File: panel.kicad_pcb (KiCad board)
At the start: 2 copper layers, 104 x 99 mm, 192 parts, among them J1 USB, J2 UART, U1 CH340X, U2 AMS1117-3.3

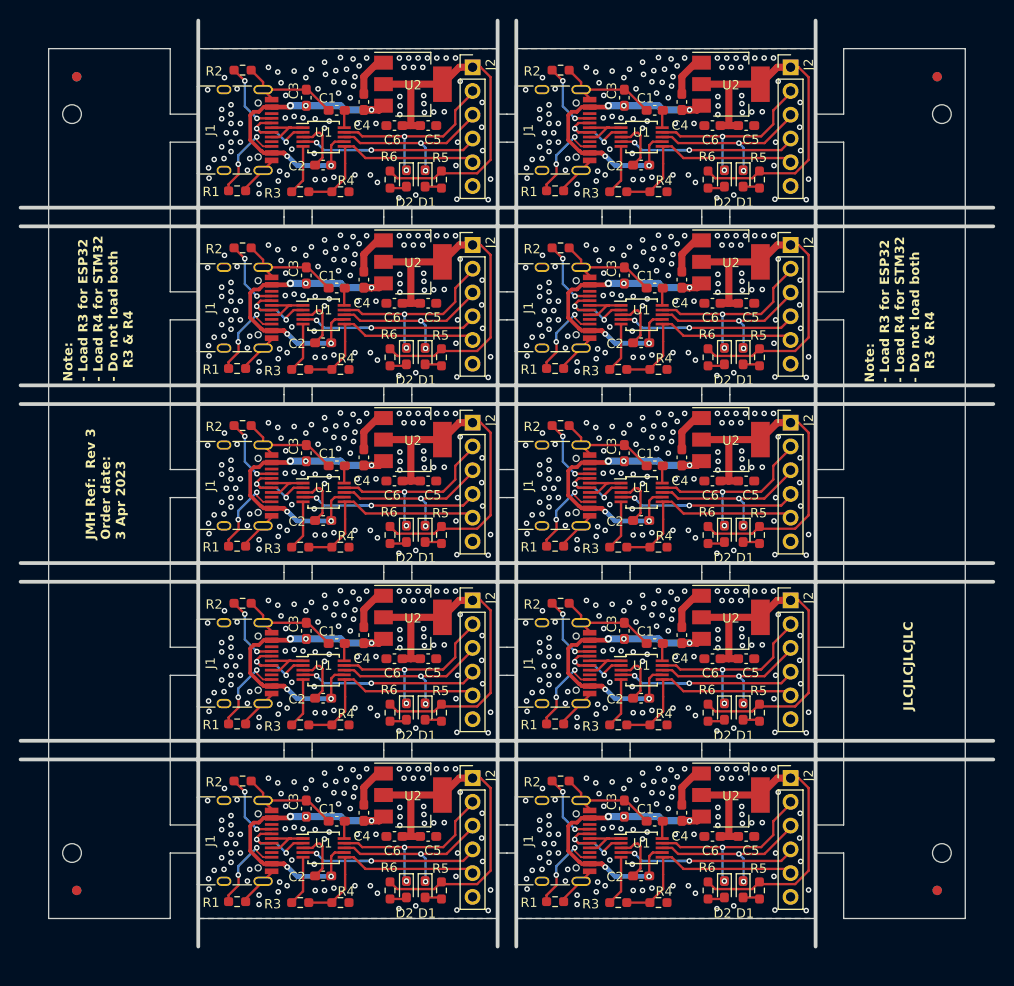
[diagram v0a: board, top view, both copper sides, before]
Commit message: Rev 5
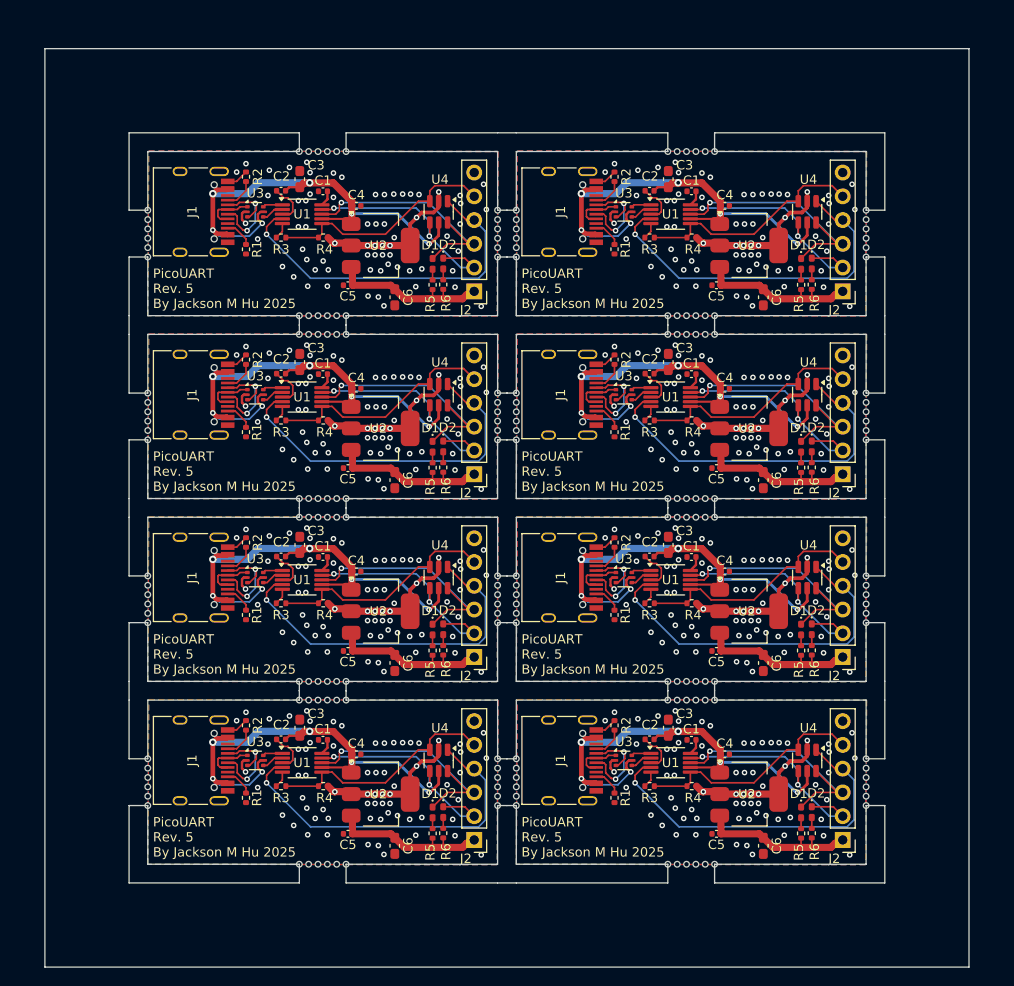
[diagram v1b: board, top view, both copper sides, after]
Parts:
- removed the C1 at (130.3, 64.6)
- removed the C1 at (130.3, 83.6)
- removed the C1 at (164.3, 102.6)
- removed the C1 at (164.3, 26.6)
- removed the C1 at (130.3, 102.6)
- removed the C1 at (130.3, 26.6)
- removed the C1 at (130.3, 45.6)
- removed the C1 at (164.3, 83.6)
- removed the C1 at (164.3, 45.6)
- removed the C1 at (164.3, 64.6)
- removed the C2 at (162.8, 70.5)
- removed the C2 at (128.8, 51.5)
- removed the C2 at (128.8, 70.5)
- removed the C2 at (162.8, 32.5)
- removed the C2 at (162.8, 108.5)
- removed the C2 at (128.8, 108.5)
- removed the C2 at (128.8, 32.5)
- removed the C2 at (128.8, 89.5)
- removed the C2 at (162.8, 51.5)
- removed the C2 at (162.8, 89.5)
- removed the C3 at (127.0, 25.2)
- removed the C3 at (127.0, 82.2)
- removed the C3 at (161.1, 44.2)
- removed the C3 at (127.0, 101.2)
- removed the C3 at (127.0, 63.2)
- removed the C3 at (161.1, 63.2)
- removed the C3 at (161.1, 82.2)
- removed the C3 at (161.1, 101.2)
- removed the C3 at (161.1, 25.2)
- removed the C3 at (127.0, 44.2)
- removed the C4 at (133.2, 25.7)
- removed the C4 at (133.2, 82.7)
- removed the C4 at (167.2, 44.7)
- removed the C4 at (133.2, 101.7)
- removed the C4 at (133.2, 63.7)
- removed the C4 at (167.2, 63.7)
- removed the C4 at (167.2, 82.7)
- removed the C4 at (167.2, 101.7)
- removed the C4 at (167.2, 25.7)
- removed the C4 at (133.2, 44.7)
- removed the C5 at (174.1, 47.2)
- removed the C5 at (140.1, 85.2)
- removed the C5 at (140.1, 104.2)
- removed the C5 at (140.1, 28.2)
- removed the C5 at (140.1, 66.2)
- removed the C5 at (174.1, 66.2)
- removed the C5 at (174.1, 85.2)
- removed the C5 at (174.1, 104.2)
- removed the C5 at (174.1, 28.2)
- removed the C5 at (140.1, 47.2)
- removed the C6 at (136.5, 28.2)
- removed the C6 at (136.5, 85.2)
- removed the C6 at (170.5, 47.2)
- removed the C6 at (136.5, 104.2)
- removed the C6 at (136.5, 66.2)
- removed the C6 at (170.5, 66.2)
- removed the C6 at (170.5, 85.2)
- removed the C6 at (170.5, 104.2)
- removed the C6 at (170.5, 28.2)
- removed the C6 at (136.5, 47.2)
- removed the D1 at (139.8, 33.9)
- removed the D1 at (139.8, 90.9)
- removed the D1 at (173.8, 52.9)
- removed the D1 at (139.8, 109.9)
- removed the D1 at (139.8, 71.9)
- removed the D1 at (173.8, 71.9)
- removed the D1 at (173.8, 90.9)
- removed the D1 at (173.8, 109.9)
- removed the D1 at (173.8, 33.9)
- removed the D1 at (139.8, 52.9)
- removed the D2 at (137.8, 33.9)
- removed the D2 at (137.8, 90.9)
- removed the D2 at (171.8, 52.9)
- removed the D2 at (137.8, 109.9)
- removed the D2 at (137.8, 71.9)
- removed the D2 at (171.8, 71.9)
- removed the D2 at (171.8, 90.9)
- removed the D2 at (171.8, 109.9)
- removed the D2 at (171.8, 33.9)
- removed the D2 at (137.8, 52.9)
- removed the J1 at (119.3, 28.7)
- removed the J1 at (119.3, 85.7)
- removed the J1 at (153.3, 47.7)
- removed the J1 at (119.3, 104.7)
- removed the J1 at (119.3, 66.7)
- removed the J1 at (153.3, 66.7)
- removed the J1 at (153.3, 85.7)
- removed the J1 at (153.3, 104.7)
- removed the J1 at (153.3, 28.7)
- removed the J1 at (119.3, 47.7)
- removed the J2 at (144.8, 22.0)
- removed the J2 at (144.8, 79.0)
- removed the J2 at (178.8, 41.0)
- removed the J2 at (144.8, 98.0)
- removed the J2 at (178.8, 22.0)
- removed the J2 at (144.8, 60.0)
- removed the J2 at (178.8, 60.0)
- removed the J2 at (178.8, 79.0)
- removed the J2 at (178.8, 98.0)
- removed the J2 at (144.8, 41.0)
- removed the R1 at (119.7, 35.2)
- removed the R1 at (119.7, 92.2)
- removed the R1 at (153.7, 54.2)
- removed the R1 at (119.7, 111.2)
- removed the R1 at (119.7, 73.2)
- removed the R1 at (153.7, 73.2)
- removed the R1 at (153.7, 92.2)
- removed the R1 at (153.7, 111.2)
- removed the R1 at (153.7, 35.2)
- removed the R1 at (119.7, 54.2)
- removed the R2 at (120.2, 22.3)
- removed the R2 at (120.2, 79.3)
- removed the R2 at (154.2, 41.3)
- removed the R2 at (120.2, 98.3)
- removed the R2 at (120.2, 60.3)
- removed the R2 at (154.2, 60.3)
- removed the R2 at (154.2, 79.3)
- removed the R2 at (154.2, 98.3)
- removed the R2 at (154.2, 22.3)
- removed the R2 at (120.2, 41.3)
- removed the R3 at (126.4, 35.3)
- removed the R3 at (126.4, 92.3)
- removed the R3 at (160.4, 54.3)
- removed the R3 at (126.4, 111.3)
- removed the R3 at (126.4, 73.3)
- removed the R3 at (160.4, 73.3)
- removed the R3 at (160.4, 92.3)
- removed the R3 at (160.4, 111.3)
- removed the R3 at (160.4, 35.3)
- removed the R3 at (126.4, 54.3)
- removed the R4 at (130.7, 35.3)
- removed the R4 at (130.7, 92.3)
- removed the R4 at (164.7, 54.3)
- removed the R4 at (130.7, 111.3)
- removed the R4 at (130.7, 73.3)
- removed the R4 at (164.7, 73.3)
- removed the R4 at (164.7, 92.3)
- removed the R4 at (164.7, 111.3)
- removed the R4 at (164.7, 35.3)
- removed the R4 at (130.7, 54.3)
- removed the R5 at (141.5, 34.0)
- removed the R5 at (141.5, 91.0)
- removed the R5 at (175.5, 53.0)
- removed the R5 at (141.5, 110.0)
- removed the R5 at (141.5, 72.0)
- removed the R5 at (175.5, 72.0)
- removed the R5 at (175.5, 91.0)
- removed the R5 at (175.5, 110.0)
- removed the R5 at (175.5, 34.0)
- removed the R5 at (141.5, 53.0)
- removed the R6 at (136.0, 34.0)
- removed the R6 at (136.0, 91.0)
- removed the R6 at (170.0, 53.0)
- removed the R6 at (136.0, 110.0)
- removed the R6 at (136.0, 72.0)
- removed the R6 at (170.0, 72.0)
- removed the R6 at (170.0, 91.0)
- removed the R6 at (170.0, 110.0)
- removed the R6 at (170.0, 34.0)
- removed the R6 at (136.0, 53.0)
- removed REF** (x8): Fiducial, Fiducial
- removed REF** (x4): NPTH, NPTH
- removed the U1 at (128.9, 105.5)
- removed the U1 at (162.9, 48.5)
- removed the U1 at (128.9, 67.5)
- removed the U1 at (162.9, 67.5)
- removed the U1 at (162.9, 86.5)
- removed the U1 at (128.9, 48.5)
- removed the U1 at (128.9, 86.5)
- removed the U1 at (162.9, 105.5)
- removed the U1 at (162.9, 29.4)
- removed the U1 at (128.9, 29.4)
- removed the U2 at (138.4, 23.8)
- removed the U2 at (138.4, 80.8)
- removed the U2 at (172.4, 42.8)
- removed the U2 at (138.4, 99.8)
- removed the U2 at (138.4, 61.8)
- removed the U2 at (172.4, 61.8)
- removed the U2 at (172.4, 80.8)
- removed the U2 at (172.4, 99.8)
- removed the U2 at (172.4, 23.8)
- removed the U2 at (138.4, 42.8)
- added C1: 100nF, Capacitor_SMD:C_0402_1005Metric, F.Cu at (128.8, 74.3)
- added C1: 100nF, Capacitor_SMD:C_0402_1005Metric, F.Cu at (128.8, 93.9)
- added C1: 100nF, Capacitor_SMD:C_0402_1005Metric, F.Cu at (168.2, 93.9)
- added C1: 100nF, Capacitor_SMD:C_0402_1005Metric, F.Cu at (168.2, 74.3)
- added C1: 100nF, Capacitor_SMD:C_0402_1005Metric, F.Cu at (168.2, 54.8)
- added C1: 100nF, Capacitor_SMD:C_0402_1005Metric, F.Cu at (168.2, 35.2)
- added C1: 100nF, Capacitor_SMD:C_0402_1005Metric, F.Cu at (128.8, 35.2)
- added C1: 100nF, Capacitor_SMD:C_0402_1005Metric, F.Cu at (128.8, 54.8)
- added C2: 100nF, Capacitor_SMD:C_0402_1005Metric, F.Cu at (163.8, 54.8)
- added C2: 100nF, Capacitor_SMD:C_0402_1005Metric, F.Cu at (163.8, 93.8)
- added C2: 100nF, Capacitor_SMD:C_0402_1005Metric, F.Cu at (163.8, 35.2)
- added C2: 100nF, Capacitor_SMD:C_0402_1005Metric, F.Cu at (124.3, 93.8)
- added C2: 100nF, Capacitor_SMD:C_0402_1005Metric, F.Cu at (124.3, 35.2)
- added C2: 100nF, Capacitor_SMD:C_0402_1005Metric, F.Cu at (124.3, 54.8)
- added C2: 100nF, Capacitor_SMD:C_0402_1005Metric, F.Cu at (163.8, 74.3)
- added C2: 100nF, Capacitor_SMD:C_0402_1005Metric, F.Cu at (124.3, 74.3)
- added C3: 10uF, Capacitor_SMD:C_0603_1608Metric_Pad1.08x0.95mm_HandSolder, F.Cu at (126.3, 53.5)
- added C3: 10uF, Capacitor_SMD:C_0603_1608Metric_Pad1.08x0.95mm_HandSolder, F.Cu at (165.8, 73.0)
- added C3: 10uF, Capacitor_SMD:C_0603_1608Metric_Pad1.08x0.95mm_HandSolder, F.Cu at (126.3, 73.0)
- added C3: 10uF, Capacitor_SMD:C_0603_1608Metric_Pad1.08x0.95mm_HandSolder, F.Cu at (165.8, 92.6)
- added C3: 10uF, Capacitor_SMD:C_0603_1608Metric_Pad1.08x0.95mm_HandSolder, F.Cu at (165.8, 34.0)
- added C3: 10uF, Capacitor_SMD:C_0603_1608Metric_Pad1.08x0.95mm_HandSolder, F.Cu at (126.3, 34.0)
- added C3: 10uF, Capacitor_SMD:C_0603_1608Metric_Pad1.08x0.95mm_HandSolder, F.Cu at (126.3, 92.6)
- added C3: 10uF, Capacitor_SMD:C_0603_1608Metric_Pad1.08x0.95mm_HandSolder, F.Cu at (165.8, 53.5)
- added C4: 0.1uF, Capacitor_SMD:C_0402_1005Metric, F.Cu at (171.8, 36.8)
- added C4: 0.1uF, Capacitor_SMD:C_0402_1005Metric, F.Cu at (132.4, 95.5)
- added C4: 0.1uF, Capacitor_SMD:C_0402_1005Metric, F.Cu at (132.4, 36.8)
- added C4: 0.1uF, Capacitor_SMD:C_0402_1005Metric, F.Cu at (132.4, 75.9)
- added C4: 0.1uF, Capacitor_SMD:C_0402_1005Metric, F.Cu at (171.8, 95.5)
- added C4: 0.1uF, Capacitor_SMD:C_0402_1005Metric, F.Cu at (171.8, 56.4)
- added C4: 0.1uF, Capacitor_SMD:C_0402_1005Metric, F.Cu at (171.8, 75.9)
- added C4: 0.1uF, Capacitor_SMD:C_0402_1005Metric, F.Cu at (132.4, 56.4)
- added C5: 0.1uF, Capacitor_SMD:C_0402_1005Metric, F.Cu at (170.9, 64.8)
- added C5: 0.1uF, Capacitor_SMD:C_0402_1005Metric, F.Cu at (131.5, 104.0)
- added C5: 0.1uF, Capacitor_SMD:C_0402_1005Metric, F.Cu at (131.5, 45.3)
- added C5: 0.1uF, Capacitor_SMD:C_0402_1005Metric, F.Cu at (170.9, 104.0)
- added C5: 0.1uF, Capacitor_SMD:C_0402_1005Metric, F.Cu at (170.9, 45.3)
- added C5: 0.1uF, Capacitor_SMD:C_0402_1005Metric, F.Cu at (131.5, 64.8)
- added C5: 0.1uF, Capacitor_SMD:C_0402_1005Metric, F.Cu at (131.5, 84.4)
- added C5: 0.1uF, Capacitor_SMD:C_0402_1005Metric, F.Cu at (170.9, 84.4)
- added C6: 10uF, Capacitor_SMD:C_0603_1608Metric_Pad1.08x0.95mm_HandSolder, F.Cu at (136.5, 105.2)
- added C6: 10uF, Capacitor_SMD:C_0603_1608Metric_Pad1.08x0.95mm_HandSolder, F.Cu at (136.5, 46.6)
- added C6: 10uF, Capacitor_SMD:C_0603_1608Metric_Pad1.08x0.95mm_HandSolder, F.Cu at (175.9, 85.7)
- added C6: 10uF, Capacitor_SMD:C_0603_1608Metric_Pad1.08x0.95mm_HandSolder, F.Cu at (136.5, 66.1)
- added C6: 10uF, Capacitor_SMD:C_0603_1608Metric_Pad1.08x0.95mm_HandSolder, F.Cu at (136.5, 85.7)
- added C6: 10uF, Capacitor_SMD:C_0603_1608Metric_Pad1.08x0.95mm_HandSolder, F.Cu at (175.9, 105.2)
- added C6: 10uF, Capacitor_SMD:C_0603_1608Metric_Pad1.08x0.95mm_HandSolder, F.Cu at (175.9, 46.6)
- added C6: 10uF, Capacitor_SMD:C_0603_1608Metric_Pad1.08x0.95mm_HandSolder, F.Cu at (175.9, 66.1)
- added D1: LED, LED_SMD:LED_0402_1005Metric_Pad0.77x0.64mm_HandSolder, F.Cu at (140.6, 82.1)
- added D1: LED, LED_SMD:LED_0402_1005Metric_Pad0.77x0.64mm_HandSolder, F.Cu at (179.9, 43.0)
- added D1: LED, LED_SMD:LED_0402_1005Metric_Pad0.77x0.64mm_HandSolder, F.Cu at (179.9, 101.7)
- added D1: LED, LED_SMD:LED_0402_1005Metric_Pad0.77x0.64mm_HandSolder, F.Cu at (140.6, 62.6)
- added D1: LED, LED_SMD:LED_0402_1005Metric_Pad0.77x0.64mm_HandSolder, F.Cu at (140.6, 101.7)
- added D1: LED, LED_SMD:LED_0402_1005Metric_Pad0.77x0.64mm_HandSolder, F.Cu at (179.9, 82.1)
- added D1: LED, LED_SMD:LED_0402_1005Metric_Pad0.77x0.64mm_HandSolder, F.Cu at (179.9, 62.6)
- added D1: LED, LED_SMD:LED_0402_1005Metric_Pad0.77x0.64mm_HandSolder, F.Cu at (140.6, 43.0)
- added D2: LED, LED_SMD:LED_0402_1005Metric_Pad0.77x0.64mm_HandSolder, F.Cu at (181.1, 101.6)
- added D2: LED, LED_SMD:LED_0402_1005Metric_Pad0.77x0.64mm_HandSolder, F.Cu at (181.1, 43.0)
- added D2: LED, LED_SMD:LED_0402_1005Metric_Pad0.77x0.64mm_HandSolder, F.Cu at (141.7, 101.6)
- added D2: LED, LED_SMD:LED_0402_1005Metric_Pad0.77x0.64mm_HandSolder, F.Cu at (141.7, 82.1)
- added D2: LED, LED_SMD:LED_0402_1005Metric_Pad0.77x0.64mm_HandSolder, F.Cu at (181.1, 62.5)
- added D2: LED, LED_SMD:LED_0402_1005Metric_Pad0.77x0.64mm_HandSolder, F.Cu at (181.1, 82.1)
- added D2: LED, LED_SMD:LED_0402_1005Metric_Pad0.77x0.64mm_HandSolder, F.Cu at (141.7, 62.5)
- added D2: LED, LED_SMD:LED_0402_1005Metric_Pad0.77x0.64mm_HandSolder, F.Cu at (141.7, 43.0)
- added J1: USB, Connector_USB:USB_C_Receptacle_HRO_TYPE-C-31-M-12, F.Cu at (114.6, 57.0)
- added J1: USB, Connector_USB:USB_C_Receptacle_HRO_TYPE-C-31-M-12, F.Cu at (154.0, 96.1)
- added J1: USB, Connector_USB:USB_C_Receptacle_HRO_TYPE-C-31-M-12, F.Cu at (154.0, 37.5)
- added J1: USB, Connector_USB:USB_C_Receptacle_HRO_TYPE-C-31-M-12, F.Cu at (154.0, 76.5)
- added J1: USB, Connector_USB:USB_C_Receptacle_HRO_TYPE-C-31-M-12, F.Cu at (154.0, 57.0)
- added J1: USB, Connector_USB:USB_C_Receptacle_HRO_TYPE-C-31-M-12, F.Cu at (114.6, 37.5)
- added J1: USB, Connector_USB:USB_C_Receptacle_HRO_TYPE-C-31-M-12, F.Cu at (114.6, 76.5)
- added J1: USB, Connector_USB:USB_C_Receptacle_HRO_TYPE-C-31-M-12, F.Cu at (114.6, 96.1)
- added J2: UART, Connector_PinHeader_2.54mm:PinHeader_1x06_P2.54mm_Vertical, F.Cu at (184.4, 46.0)
- added J2: UART, Connector_PinHeader_2.54mm:PinHeader_1x06_P2.54mm_Vertical, F.Cu at (184.4, 65.5)
- added J2: UART, Connector_PinHeader_2.54mm:PinHeader_1x06_P2.54mm_Vertical, F.Cu at (145.0, 104.6)
- added J2: UART, Connector_PinHeader_2.54mm:PinHeader_1x06_P2.54mm_Vertical, F.Cu at (145.0, 85.0)
- added J2: UART, Connector_PinHeader_2.54mm:PinHeader_1x06_P2.54mm_Vertical, F.Cu at (145.0, 46.0)
- added J2: UART, Connector_PinHeader_2.54mm:PinHeader_1x06_P2.54mm_Vertical, F.Cu at (184.4, 85.0)
- added J2: UART, Connector_PinHeader_2.54mm:PinHeader_1x06_P2.54mm_Vertical, F.Cu at (145.0, 65.5)
- added J2: UART, Connector_PinHeader_2.54mm:PinHeader_1x06_P2.54mm_Vertical, F.Cu at (184.4, 104.6)
- added KiKit_MB_10_1: NPTH, NPTH, F.Cu at (147.5, 56.8)
- added KiKit_MB_10_2: NPTH, NPTH, F.Cu at (147.5, 57.8)
- added KiKit_MB_10_3: NPTH, NPTH, F.Cu at (147.5, 58.8)
- added KiKit_MB_10_4: NPTH, NPTH, F.Cu at (147.5, 59.8)
- added KiKit_MB_10_5: NPTH, NPTH, F.Cu at (147.5, 60.8)
- added KiKit_MB_10_6: NPTH, NPTH, F.Cu at (147.5, 61.8)
- added KiKit_MB_11_1: NPTH, NPTH, F.Cu at (126.3, 50.5)
- added KiKit_MB_11_2: NPTH, NPTH, F.Cu at (127.3, 50.5)
- added KiKit_MB_11_3: NPTH, NPTH, F.Cu at (128.3, 50.5)
- added KiKit_MB_11_4: NPTH, NPTH, F.Cu at (129.3, 50.5)
- added KiKit_MB_11_5: NPTH, NPTH, F.Cu at (130.3, 50.5)
- added KiKit_MB_11_6: NPTH, NPTH, F.Cu at (131.3, 50.5)
- added KiKit_MB_12_1: NPTH, NPTH, F.Cu at (131.3, 68.1)
- added KiKit_MB_12_2: NPTH, NPTH, F.Cu at (130.3, 68.1)
- added KiKit_MB_12_3: NPTH, NPTH, F.Cu at (129.3, 68.1)
- added KiKit_MB_12_4: NPTH, NPTH, F.Cu at (128.3, 68.1)
- added KiKit_MB_12_5: NPTH, NPTH, F.Cu at (127.3, 68.1)
- added KiKit_MB_12_6: NPTH, NPTH, F.Cu at (126.3, 68.1)
- added KiKit_MB_13_1: NPTH, NPTH, F.Cu at (149.5, 61.8)
- added KiKit_MB_13_2: NPTH, NPTH, F.Cu at (149.5, 60.8)
- added KiKit_MB_13_3: NPTH, NPTH, F.Cu at (149.5, 59.8)
- added KiKit_MB_13_4: NPTH, NPTH, F.Cu at (149.5, 58.8)
- added KiKit_MB_13_5: NPTH, NPTH, F.Cu at (149.5, 57.8)
- added KiKit_MB_13_6: NPTH, NPTH, F.Cu at (149.5, 56.8)
- added KiKit_MB_14_1: NPTH, NPTH, F.Cu at (186.9, 56.8)
- added KiKit_MB_14_2: NPTH, NPTH, F.Cu at (186.9, 57.8)
- added KiKit_MB_14_3: NPTH, NPTH, F.Cu at (186.9, 58.8)
- added KiKit_MB_14_4: NPTH, NPTH, F.Cu at (186.9, 59.8)
- added KiKit_MB_14_5: NPTH, NPTH, F.Cu at (186.9, 60.8)
- added KiKit_MB_14_6: NPTH, NPTH, F.Cu at (186.9, 61.8)
- added KiKit_MB_15_1: NPTH, NPTH, F.Cu at (165.7, 50.5)
- added KiKit_MB_15_2: NPTH, NPTH, F.Cu at (166.7, 50.5)
- added KiKit_MB_15_3: NPTH, NPTH, F.Cu at (167.7, 50.5)
- added KiKit_MB_15_4: NPTH, NPTH, F.Cu at (168.7, 50.5)
- added KiKit_MB_15_5: NPTH, NPTH, F.Cu at (169.7, 50.5)
- added KiKit_MB_15_6: NPTH, NPTH, F.Cu at (170.7, 50.5)
- added KiKit_MB_16_1: NPTH, NPTH, F.Cu at (170.7, 68.1)
- added KiKit_MB_16_2: NPTH, NPTH, F.Cu at (169.7, 68.1)
- added KiKit_MB_16_3: NPTH, NPTH, F.Cu at (168.7, 68.1)
- added KiKit_MB_16_4: NPTH, NPTH, F.Cu at (167.7, 68.1)
- added KiKit_MB_16_5: NPTH, NPTH, F.Cu at (166.7, 68.1)
- added KiKit_MB_16_6: NPTH, NPTH, F.Cu at (165.7, 68.1)
- added KiKit_MB_17_1: NPTH, NPTH, F.Cu at (110.1, 81.4)
- added KiKit_MB_17_2: NPTH, NPTH, F.Cu at (110.1, 80.4)
- added KiKit_MB_17_3: NPTH, NPTH, F.Cu at (110.1, 79.4)
- added KiKit_MB_17_4: NPTH, NPTH, F.Cu at (110.1, 78.4)
- added KiKit_MB_17_5: NPTH, NPTH, F.Cu at (110.1, 77.4)
- added KiKit_MB_17_6: NPTH, NPTH, F.Cu at (110.1, 76.4)
- added KiKit_MB_18_1: NPTH, NPTH, F.Cu at (147.5, 76.4)
- added KiKit_MB_18_2: NPTH, NPTH, F.Cu at (147.5, 77.4)
- added KiKit_MB_18_3: NPTH, NPTH, F.Cu at (147.5, 78.4)
- added KiKit_MB_18_4: NPTH, NPTH, F.Cu at (147.5, 79.4)
- added KiKit_MB_18_5: NPTH, NPTH, F.Cu at (147.5, 80.4)
- added KiKit_MB_18_6: NPTH, NPTH, F.Cu at (147.5, 81.4)
- added KiKit_MB_19_1: NPTH, NPTH, F.Cu at (126.3, 70.1)
- added KiKit_MB_19_2: NPTH, NPTH, F.Cu at (127.3, 70.1)
- added KiKit_MB_19_3: NPTH, NPTH, F.Cu at (128.3, 70.1)
- added KiKit_MB_19_4: NPTH, NPTH, F.Cu at (129.3, 70.1)
- added KiKit_MB_19_5: NPTH, NPTH, F.Cu at (130.3, 70.1)
- added KiKit_MB_19_6: NPTH, NPTH, F.Cu at (131.3, 70.1)
- added KiKit_MB_1_1: NPTH, NPTH, F.Cu at (110.1, 42.3)
- added KiKit_MB_1_2: NPTH, NPTH, F.Cu at (110.1, 41.3)
- added KiKit_MB_1_3: NPTH, NPTH, F.Cu at (110.1, 40.3)
- added KiKit_MB_1_4: NPTH, NPTH, F.Cu at (110.1, 39.3)
- added KiKit_MB_1_5: NPTH, NPTH, F.Cu at (110.1, 38.3)
- added KiKit_MB_1_6: NPTH, NPTH, F.Cu at (110.1, 37.3)
- added KiKit_MB_20_1: NPTH, NPTH, F.Cu at (131.3, 87.7)
- added KiKit_MB_20_2: NPTH, NPTH, F.Cu at (130.3, 87.7)
- added KiKit_MB_20_3: NPTH, NPTH, F.Cu at (129.3, 87.7)
- added KiKit_MB_20_4: NPTH, NPTH, F.Cu at (128.3, 87.7)
- added KiKit_MB_20_5: NPTH, NPTH, F.Cu at (127.3, 87.7)
- added KiKit_MB_20_6: NPTH, NPTH, F.Cu at (126.3, 87.7)
- added KiKit_MB_21_1: NPTH, NPTH, F.Cu at (149.5, 81.4)
- added KiKit_MB_21_2: NPTH, NPTH, F.Cu at (149.5, 80.4)
- added KiKit_MB_21_3: NPTH, NPTH, F.Cu at (149.5, 79.4)
- added KiKit_MB_21_4: NPTH, NPTH, F.Cu at (149.5, 78.4)
- added KiKit_MB_21_5: NPTH, NPTH, F.Cu at (149.5, 77.4)
- added KiKit_MB_21_6: NPTH, NPTH, F.Cu at (149.5, 76.4)
- added KiKit_MB_22_1: NPTH, NPTH, F.Cu at (186.9, 76.4)
- added KiKit_MB_22_2: NPTH, NPTH, F.Cu at (186.9, 77.4)
- added KiKit_MB_22_3: NPTH, NPTH, F.Cu at (186.9, 78.4)
- added KiKit_MB_22_4: NPTH, NPTH, F.Cu at (186.9, 79.4)
- added KiKit_MB_22_5: NPTH, NPTH, F.Cu at (186.9, 80.4)
- added KiKit_MB_22_6: NPTH, NPTH, F.Cu at (186.9, 81.4)
- added KiKit_MB_23_1: NPTH, NPTH, F.Cu at (165.7, 70.1)
- added KiKit_MB_23_2: NPTH, NPTH, F.Cu at (166.7, 70.1)
- added KiKit_MB_23_3: NPTH, NPTH, F.Cu at (167.7, 70.1)
- added KiKit_MB_23_4: NPTH, NPTH, F.Cu at (168.7, 70.1)
- added KiKit_MB_23_5: NPTH, NPTH, F.Cu at (169.7, 70.1)
- added KiKit_MB_23_6: NPTH, NPTH, F.Cu at (170.7, 70.1)
- added KiKit_MB_24_1: NPTH, NPTH, F.Cu at (170.7, 87.7)
- added KiKit_MB_24_2: NPTH, NPTH, F.Cu at (169.7, 87.7)
- added KiKit_MB_24_3: NPTH, NPTH, F.Cu at (168.7, 87.7)
- added KiKit_MB_24_4: NPTH, NPTH, F.Cu at (167.7, 87.7)
- added KiKit_MB_24_5: NPTH, NPTH, F.Cu at (166.7, 87.7)
- added KiKit_MB_24_6: NPTH, NPTH, F.Cu at (165.7, 87.7)
- added KiKit_MB_25_1: NPTH, NPTH, F.Cu at (110.1, 100.9)
- added KiKit_MB_25_2: NPTH, NPTH, F.Cu at (110.1, 99.9)
- added KiKit_MB_25_3: NPTH, NPTH, F.Cu at (110.1, 98.9)
- added KiKit_MB_25_4: NPTH, NPTH, F.Cu at (110.1, 97.9)
- added KiKit_MB_25_5: NPTH, NPTH, F.Cu at (110.1, 96.9)
- added KiKit_MB_25_6: NPTH, NPTH, F.Cu at (110.1, 95.9)
- added KiKit_MB_26_1: NPTH, NPTH, F.Cu at (147.5, 95.9)
- added KiKit_MB_26_2: NPTH, NPTH, F.Cu at (147.5, 96.9)
- added KiKit_MB_26_3: NPTH, NPTH, F.Cu at (147.5, 97.9)
- added KiKit_MB_26_4: NPTH, NPTH, F.Cu at (147.5, 98.9)
- added KiKit_MB_26_5: NPTH, NPTH, F.Cu at (147.5, 99.9)
- added KiKit_MB_26_6: NPTH, NPTH, F.Cu at (147.5, 100.9)
- added KiKit_MB_27_1: NPTH, NPTH, F.Cu at (126.3, 89.7)
- added KiKit_MB_27_2: NPTH, NPTH, F.Cu at (127.3, 89.7)
- added KiKit_MB_27_3: NPTH, NPTH, F.Cu at (128.3, 89.7)
- added KiKit_MB_27_4: NPTH, NPTH, F.Cu at (129.3, 89.7)
- added KiKit_MB_27_5: NPTH, NPTH, F.Cu at (130.3, 89.7)
- added KiKit_MB_27_6: NPTH, NPTH, F.Cu at (131.3, 89.7)
- added KiKit_MB_28_1: NPTH, NPTH, F.Cu at (131.3, 107.2)
- added KiKit_MB_28_2: NPTH, NPTH, F.Cu at (130.3, 107.2)
- added KiKit_MB_28_3: NPTH, NPTH, F.Cu at (129.3, 107.2)
- added KiKit_MB_28_4: NPTH, NPTH, F.Cu at (128.3, 107.2)
- added KiKit_MB_28_5: NPTH, NPTH, F.Cu at (127.3, 107.2)
- added KiKit_MB_28_6: NPTH, NPTH, F.Cu at (126.3, 107.2)
- added KiKit_MB_29_1: NPTH, NPTH, F.Cu at (149.5, 100.9)
- added KiKit_MB_29_2: NPTH, NPTH, F.Cu at (149.5, 99.9)
- added KiKit_MB_29_3: NPTH, NPTH, F.Cu at (149.5, 98.9)
- added KiKit_MB_29_4: NPTH, NPTH, F.Cu at (149.5, 97.9)
- added KiKit_MB_29_5: NPTH, NPTH, F.Cu at (149.5, 96.9)
- added KiKit_MB_29_6: NPTH, NPTH, F.Cu at (149.5, 95.9)
- added KiKit_MB_2_1: NPTH, NPTH, F.Cu at (147.5, 37.3)
- added KiKit_MB_2_2: NPTH, NPTH, F.Cu at (147.5, 38.3)
- added KiKit_MB_2_3: NPTH, NPTH, F.Cu at (147.5, 39.3)
- added KiKit_MB_2_4: NPTH, NPTH, F.Cu at (147.5, 40.3)
- added KiKit_MB_2_5: NPTH, NPTH, F.Cu at (147.5, 41.3)
- added KiKit_MB_2_6: NPTH, NPTH, F.Cu at (147.5, 42.3)
- added KiKit_MB_30_1: NPTH, NPTH, F.Cu at (186.9, 95.9)
- added KiKit_MB_30_2: NPTH, NPTH, F.Cu at (186.9, 96.9)
- added KiKit_MB_30_3: NPTH, NPTH, F.Cu at (186.9, 97.9)
- added KiKit_MB_30_4: NPTH, NPTH, F.Cu at (186.9, 98.9)
- added KiKit_MB_30_5: NPTH, NPTH, F.Cu at (186.9, 99.9)
- added KiKit_MB_30_6: NPTH, NPTH, F.Cu at (186.9, 100.9)
- added KiKit_MB_31_1: NPTH, NPTH, F.Cu at (165.7, 89.7)
- added KiKit_MB_31_2: NPTH, NPTH, F.Cu at (166.7, 89.7)
- added KiKit_MB_31_3: NPTH, NPTH, F.Cu at (167.7, 89.7)
- added KiKit_MB_31_4: NPTH, NPTH, F.Cu at (168.7, 89.7)
- added KiKit_MB_31_5: NPTH, NPTH, F.Cu at (169.7, 89.7)
- added KiKit_MB_31_6: NPTH, NPTH, F.Cu at (170.7, 89.7)
- added KiKit_MB_32_1: NPTH, NPTH, F.Cu at (170.7, 107.2)
- added KiKit_MB_32_2: NPTH, NPTH, F.Cu at (169.7, 107.2)
- added KiKit_MB_32_3: NPTH, NPTH, F.Cu at (168.7, 107.2)
- added KiKit_MB_32_4: NPTH, NPTH, F.Cu at (167.7, 107.2)
- added KiKit_MB_32_5: NPTH, NPTH, F.Cu at (166.7, 107.2)
- added KiKit_MB_32_6: NPTH, NPTH, F.Cu at (165.7, 107.2)
- added KiKit_MB_3_1: NPTH, NPTH, F.Cu at (126.3, 31.0)
- added KiKit_MB_3_2: NPTH, NPTH, F.Cu at (127.3, 31.0)
- added KiKit_MB_3_3: NPTH, NPTH, F.Cu at (128.3, 31.0)
- added KiKit_MB_3_4: NPTH, NPTH, F.Cu at (129.3, 31.0)
- added KiKit_MB_3_5: NPTH, NPTH, F.Cu at (130.3, 31.0)
- added KiKit_MB_3_6: NPTH, NPTH, F.Cu at (131.3, 31.0)
- added KiKit_MB_4_1: NPTH, NPTH, F.Cu at (131.3, 48.5)
- added KiKit_MB_4_2: NPTH, NPTH, F.Cu at (130.3, 48.5)
- added KiKit_MB_4_3: NPTH, NPTH, F.Cu at (129.3, 48.5)
- added KiKit_MB_4_4: NPTH, NPTH, F.Cu at (128.3, 48.5)
- added KiKit_MB_4_5: NPTH, NPTH, F.Cu at (127.3, 48.5)
- added KiKit_MB_4_6: NPTH, NPTH, F.Cu at (126.3, 48.5)
- added KiKit_MB_5_1: NPTH, NPTH, F.Cu at (149.5, 42.3)
- added KiKit_MB_5_2: NPTH, NPTH, F.Cu at (149.5, 41.3)
- added KiKit_MB_5_3: NPTH, NPTH, F.Cu at (149.5, 40.3)
- added KiKit_MB_5_4: NPTH, NPTH, F.Cu at (149.5, 39.3)
- added KiKit_MB_5_5: NPTH, NPTH, F.Cu at (149.5, 38.3)
- added KiKit_MB_5_6: NPTH, NPTH, F.Cu at (149.5, 37.3)
- added KiKit_MB_6_1: NPTH, NPTH, F.Cu at (186.9, 37.3)
- added KiKit_MB_6_2: NPTH, NPTH, F.Cu at (186.9, 38.3)
- added KiKit_MB_6_3: NPTH, NPTH, F.Cu at (186.9, 39.3)
- added KiKit_MB_6_4: NPTH, NPTH, F.Cu at (186.9, 40.3)
- added KiKit_MB_6_5: NPTH, NPTH, F.Cu at (186.9, 41.3)
- added KiKit_MB_6_6: NPTH, NPTH, F.Cu at (186.9, 42.3)
- added KiKit_MB_7_1: NPTH, NPTH, F.Cu at (165.7, 31.0)
- added KiKit_MB_7_2: NPTH, NPTH, F.Cu at (166.7, 31.0)
- added KiKit_MB_7_3: NPTH, NPTH, F.Cu at (167.7, 31.0)
- added KiKit_MB_7_4: NPTH, NPTH, F.Cu at (168.7, 31.0)
- added KiKit_MB_7_5: NPTH, NPTH, F.Cu at (169.7, 31.0)
- added KiKit_MB_7_6: NPTH, NPTH, F.Cu at (170.7, 31.0)
- added KiKit_MB_8_1: NPTH, NPTH, F.Cu at (170.7, 48.5)
- added KiKit_MB_8_2: NPTH, NPTH, F.Cu at (169.7, 48.5)
- added KiKit_MB_8_3: NPTH, NPTH, F.Cu at (168.7, 48.5)
- added KiKit_MB_8_4: NPTH, NPTH, F.Cu at (167.7, 48.5)
- added KiKit_MB_8_5: NPTH, NPTH, F.Cu at (166.7, 48.5)
- added KiKit_MB_8_6: NPTH, NPTH, F.Cu at (165.7, 48.5)
- added KiKit_MB_9_1: NPTH, NPTH, F.Cu at (110.1, 61.8)
- added KiKit_MB_9_2: NPTH, NPTH, F.Cu at (110.1, 60.8)
- added KiKit_MB_9_3: NPTH, NPTH, F.Cu at (110.1, 59.8)
- added KiKit_MB_9_4: NPTH, NPTH, F.Cu at (110.1, 58.8)
- added KiKit_MB_9_5: NPTH, NPTH, F.Cu at (110.1, 57.8)
- added KiKit_MB_9_6: NPTH, NPTH, F.Cu at (110.1, 56.8)
- added R1: 5.11k, Resistor_SMD:R_0402_1005Metric, F.Cu at (160.0, 41.5)
- added R1: 5.11k, Resistor_SMD:R_0402_1005Metric, F.Cu at (160.0, 100.1)
- added R1: 5.11k, Resistor_SMD:R_0402_1005Metric, F.Cu at (160.0, 80.5)
- added R1: 5.11k, Resistor_SMD:R_0402_1005Metric, F.Cu at (120.6, 100.1)
- added R1: 5.11k, Resistor_SMD:R_0402_1005Metric, F.Cu at (120.6, 80.5)
- added R1: 5.11k, Resistor_SMD:R_0402_1005Metric, F.Cu at (120.6, 41.5)
- added R1: 5.11k, Resistor_SMD:R_0402_1005Metric, F.Cu at (160.0, 61.0)
- added R1: 5.11k, Resistor_SMD:R_0402_1005Metric, F.Cu at (120.6, 61.0)
- added R2: 5.11k, Resistor_SMD:R_0402_1005Metric, F.Cu at (160.0, 92.3)
- added R2: 5.11k, Resistor_SMD:R_0402_1005Metric, F.Cu at (160.0, 72.8)
- added R2: 5.11k, Resistor_SMD:R_0402_1005Metric, F.Cu at (120.6, 33.7)
- added R2: 5.11k, Resistor_SMD:R_0402_1005Metric, F.Cu at (160.0, 33.7)
- added R2: 5.11k, Resistor_SMD:R_0402_1005Metric, F.Cu at (120.6, 92.3)
- added R2: 5.11k, Resistor_SMD:R_0402_1005Metric, F.Cu at (120.6, 72.8)
- added R2: 5.11k, Resistor_SMD:R_0402_1005Metric, F.Cu at (120.6, 53.2)
- added R2: 5.11k, Resistor_SMD:R_0402_1005Metric, F.Cu at (160.0, 53.2)
- added R3: 4.7k, Resistor_SMD:R_0402_1005Metric, F.Cu at (124.3, 40.2)
- added R3: 4.7k, Resistor_SMD:R_0402_1005Metric, F.Cu at (124.3, 98.8)
- added R3: 4.7k, Resistor_SMD:R_0402_1005Metric, F.Cu at (163.8, 98.8)
- added R3: 4.7k, Resistor_SMD:R_0402_1005Metric, F.Cu at (163.8, 40.2)
- added R3: 4.7k, Resistor_SMD:R_0402_1005Metric, F.Cu at (124.3, 79.3)
- added R3: 4.7k, Resistor_SMD:R_0402_1005Metric, F.Cu at (163.8, 59.8)
- added R3: 4.7k, Resistor_SMD:R_0402_1005Metric, F.Cu at (124.3, 59.8)
- added R3: 4.7k, Resistor_SMD:R_0402_1005Metric, F.Cu at (163.8, 79.3)
- added R4: 4.7k, Resistor_SMD:R_0402_1005Metric, F.Cu at (128.9, 59.8)
- added R4: 4.7k, Resistor_SMD:R_0402_1005Metric, F.Cu at (128.9, 79.3)
- added R4: 4.7k, Resistor_SMD:R_0402_1005Metric, F.Cu at (168.3, 40.2)
- added R4: 4.7k, Resistor_SMD:R_0402_1005Metric, F.Cu at (168.3, 59.8)
- added R4: 4.7k, Resistor_SMD:R_0402_1005Metric, F.Cu at (128.9, 98.8)
- added R4: 4.7k, Resistor_SMD:R_0402_1005Metric, F.Cu at (168.3, 79.3)
- added R4: 4.7k, Resistor_SMD:R_0402_1005Metric, F.Cu at (128.9, 40.2)
- added R4: 4.7k, Resistor_SMD:R_0402_1005Metric, F.Cu at (168.3, 98.8)
- added R5: 1k, Resistor_SMD:R_0402_1005Metric, F.Cu at (179.9, 45.2)
- added R5: 1k, Resistor_SMD:R_0402_1005Metric, F.Cu at (179.9, 64.8)
- added R5: 1k, Resistor_SMD:R_0402_1005Metric, F.Cu at (140.6, 103.9)
- added R5: 1k, Resistor_SMD:R_0402_1005Metric, F.Cu at (140.6, 64.8)
- added R5: 1k, Resistor_SMD:R_0402_1005Metric, F.Cu at (179.9, 84.3)
- added R5: 1k, Resistor_SMD:R_0402_1005Metric, F.Cu at (140.6, 45.2)
- added R5: 1k, Resistor_SMD:R_0402_1005Metric, F.Cu at (140.6, 84.3)
- added R5: 1k, Resistor_SMD:R_0402_1005Metric, F.Cu at (179.9, 103.9)
- added R6: 1k, Resistor_SMD:R_0402_1005Metric, F.Cu at (141.7, 84.3)
- added R6: 1k, Resistor_SMD:R_0402_1005Metric, F.Cu at (181.1, 84.3)
- added R6: 1k, Resistor_SMD:R_0402_1005Metric, F.Cu at (141.7, 64.8)
- added R6: 1k, Resistor_SMD:R_0402_1005Metric, F.Cu at (181.1, 64.8)
- added R6: 1k, Resistor_SMD:R_0402_1005Metric, F.Cu at (141.7, 45.2)
- added R6: 1k, Resistor_SMD:R_0402_1005Metric, F.Cu at (181.1, 45.2)
- added R6: 1k, Resistor_SMD:R_0402_1005Metric, F.Cu at (181.1, 103.9)
- added R6: 1k, Resistor_SMD:R_0402_1005Metric, F.Cu at (141.7, 103.9)
- added U1: CH340X, Package_SO:MSOP-10_3x3mm_P0.5mm, F.Cu at (126.6, 76.8)
- added U1: CH340X, Package_SO:MSOP-10_3x3mm_P0.5mm, F.Cu at (126.6, 37.7)
- added U1: CH340X, Package_SO:MSOP-10_3x3mm_P0.5mm, F.Cu at (126.6, 57.2)
- added U1: CH340X, Package_SO:MSOP-10_3x3mm_P0.5mm, F.Cu at (166.0, 57.2)
- added U1: CH340X, Package_SO:MSOP-10_3x3mm_P0.5mm, F.Cu at (166.0, 37.7)
- added U1: CH340X, Package_SO:MSOP-10_3x3mm_P0.5mm, F.Cu at (166.0, 96.3)
- added U1: CH340X, Package_SO:MSOP-10_3x3mm_P0.5mm, F.Cu at (126.6, 96.3)
- added U1: CH340X, Package_SO:MSOP-10_3x3mm_P0.5mm, F.Cu at (166.0, 76.8)
- added U2: AP7361C-33E, Package_TO_SOT_SMD:SOT-223-3_TabPin2, F.Cu at (174.4, 60.6)
- added U2: AP7361C-33E, Package_TO_SOT_SMD:SOT-223-3_TabPin2, F.Cu at (135.0, 41.0)
- added U2: AP7361C-33E, Package_TO_SOT_SMD:SOT-223-3_TabPin2, F.Cu at (135.0, 99.7)
- added U2: AP7361C-33E, Package_TO_SOT_SMD:SOT-223-3_TabPin2, F.Cu at (174.4, 80.2)
- added U2: AP7361C-33E, Package_TO_SOT_SMD:SOT-223-3_TabPin2, F.Cu at (135.0, 80.2)
- added U2: AP7361C-33E, Package_TO_SOT_SMD:SOT-223-3_TabPin2, F.Cu at (174.4, 41.0)
- added U2: AP7361C-33E, Package_TO_SOT_SMD:SOT-223-3_TabPin2, F.Cu at (135.0, 60.6)
- added U2: AP7361C-33E, Package_TO_SOT_SMD:SOT-223-3_TabPin2, F.Cu at (174.4, 99.7)
- added U3: USBLC6-2P6, Package_TO_SOT_SMD:SOT-666, F.Cu at (121.6, 96.1)
- added U3: USBLC6-2P6, Package_TO_SOT_SMD:SOT-666, F.Cu at (121.6, 37.5)
- added U3: USBLC6-2P6, Package_TO_SOT_SMD:SOT-666, F.Cu at (161.0, 37.5)
- added U3: USBLC6-2P6, Package_TO_SOT_SMD:SOT-666, F.Cu at (161.0, 57.0)
- added U3: USBLC6-2P6, Package_TO_SOT_SMD:SOT-666, F.Cu at (161.0, 96.1)
- added U3: USBLC6-2P6, Package_TO_SOT_SMD:SOT-666, F.Cu at (121.6, 57.0)
- added U3: USBLC6-2P6, Package_TO_SOT_SMD:SOT-666, F.Cu at (161.0, 76.5)
- added U3: USBLC6-2P6, Package_TO_SOT_SMD:SOT-666, F.Cu at (121.6, 76.5)
- added U4: USBLC6-4SC6, Package_TO_SOT_SMD:SOT-23-6, F.Cu at (141.2, 76.5)
- added U4: USBLC6-4SC6, Package_TO_SOT_SMD:SOT-23-6, F.Cu at (180.6, 96.1)
- added U4: USBLC6-4SC6, Package_TO_SOT_SMD:SOT-23-6, F.Cu at (180.6, 76.5)
- added U4: USBLC6-4SC6, Package_TO_SOT_SMD:SOT-23-6, F.Cu at (180.6, 57.0)
- added U4: USBLC6-4SC6, Package_TO_SOT_SMD:SOT-23-6, F.Cu at (141.2, 96.1)
- added U4: USBLC6-4SC6, Package_TO_SOT_SMD:SOT-23-6, F.Cu at (180.6, 37.5)
- added U4: USBLC6-4SC6, Package_TO_SOT_SMD:SOT-23-6, F.Cu at (141.2, 57.0)
- added U4: USBLC6-4SC6, Package_TO_SOT_SMD:SOT-23-6, F.Cu at (141.2, 37.5)
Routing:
- net Board_9-+3V3: track 39.9 -> 0.00 mm
- net Board_8-+3V3: track 39.9 -> 0.00 mm
- net Board_8-+5V: track 32.0 -> 0.00 mm, vias 5 -> 0
- net Board_9-+5V: track 32.0 -> 0.00 mm, vias 5 -> 0
- net Board_9-GND: track 26.8 -> 0.00 mm, vias 93 -> 0
- net Board_8-GND: track 26.8 -> 0.00 mm, vias 93 -> 0
- net Board_9-BOOT: track 22.5 -> 0.00 mm
- net Board_8-BOOT: track 22.5 -> 0.00 mm
- net Board_1-+3V3: track 39.9 -> 18.0 mm
- net Board_5-+3V3: track 39.9 -> 18.0 mm
- net Board_3-+3V3: track 39.9 -> 18.0 mm
- net Board_0-+3V3: track 39.9 -> 18.0 mm
- net Board_4-+3V3: track 39.9 -> 18.0 mm
- net Board_2-+3V3: track 39.9 -> 18.0 mm
- net Board_7-+3V3: track 39.9 -> 18.0 mm
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- removed copper zone on B.Cu, net Board_8-GND
- removed copper zone on F.Cu, net Board_8-GND
- removed copper zone on B.Cu, net Board_9-GND
- removed copper zone on F.Cu, net Board_9-GND
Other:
- board size 104 x 99 mm -> 98.8 x 98.2 mm
- board text added: "GND BOOT RST TxD RxD +3v3"
- board text added: "PREVIEW ONLY. PANEL SAVED IN /Users/hu/HardwareProjects/picouart/panel-rev5.kicad_pcb"
- board text added: "PicoUART Rev. 5 By Jackson M Hu 2025"
- board text removed: "3v3 RxD TxD RST BOOT GND"
- board text removed: "By Jackson M Hu (C) 2023"
- board text removed: "JLCJLCJLCJLC"
- board text removed: "JMH Ref: Rev 3 Order date: 3 Apr 2023"
- board text removed: "Note: - Load R3 for ESP32 - Load R4 for STM32 - Do not load both R3 & R4"
- board text removed: "PicoUART Rev 3"
- board text removed: "V-CUT"
